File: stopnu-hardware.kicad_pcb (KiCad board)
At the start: 4 copper layers, 150 x 128 mm, 48 parts, among them CN1 SM04B-SRSS-TB (LF)(SN), CN2 OQ0232510000G, CN3 OQ0232510000G, CN4 OQ0232510000G, U1 WIFI_KIT_32__V3_, U2 74HCT1G125GW-Q100H, U5 LTV-817S, U6 LTV-817S, U7 LTV-817S

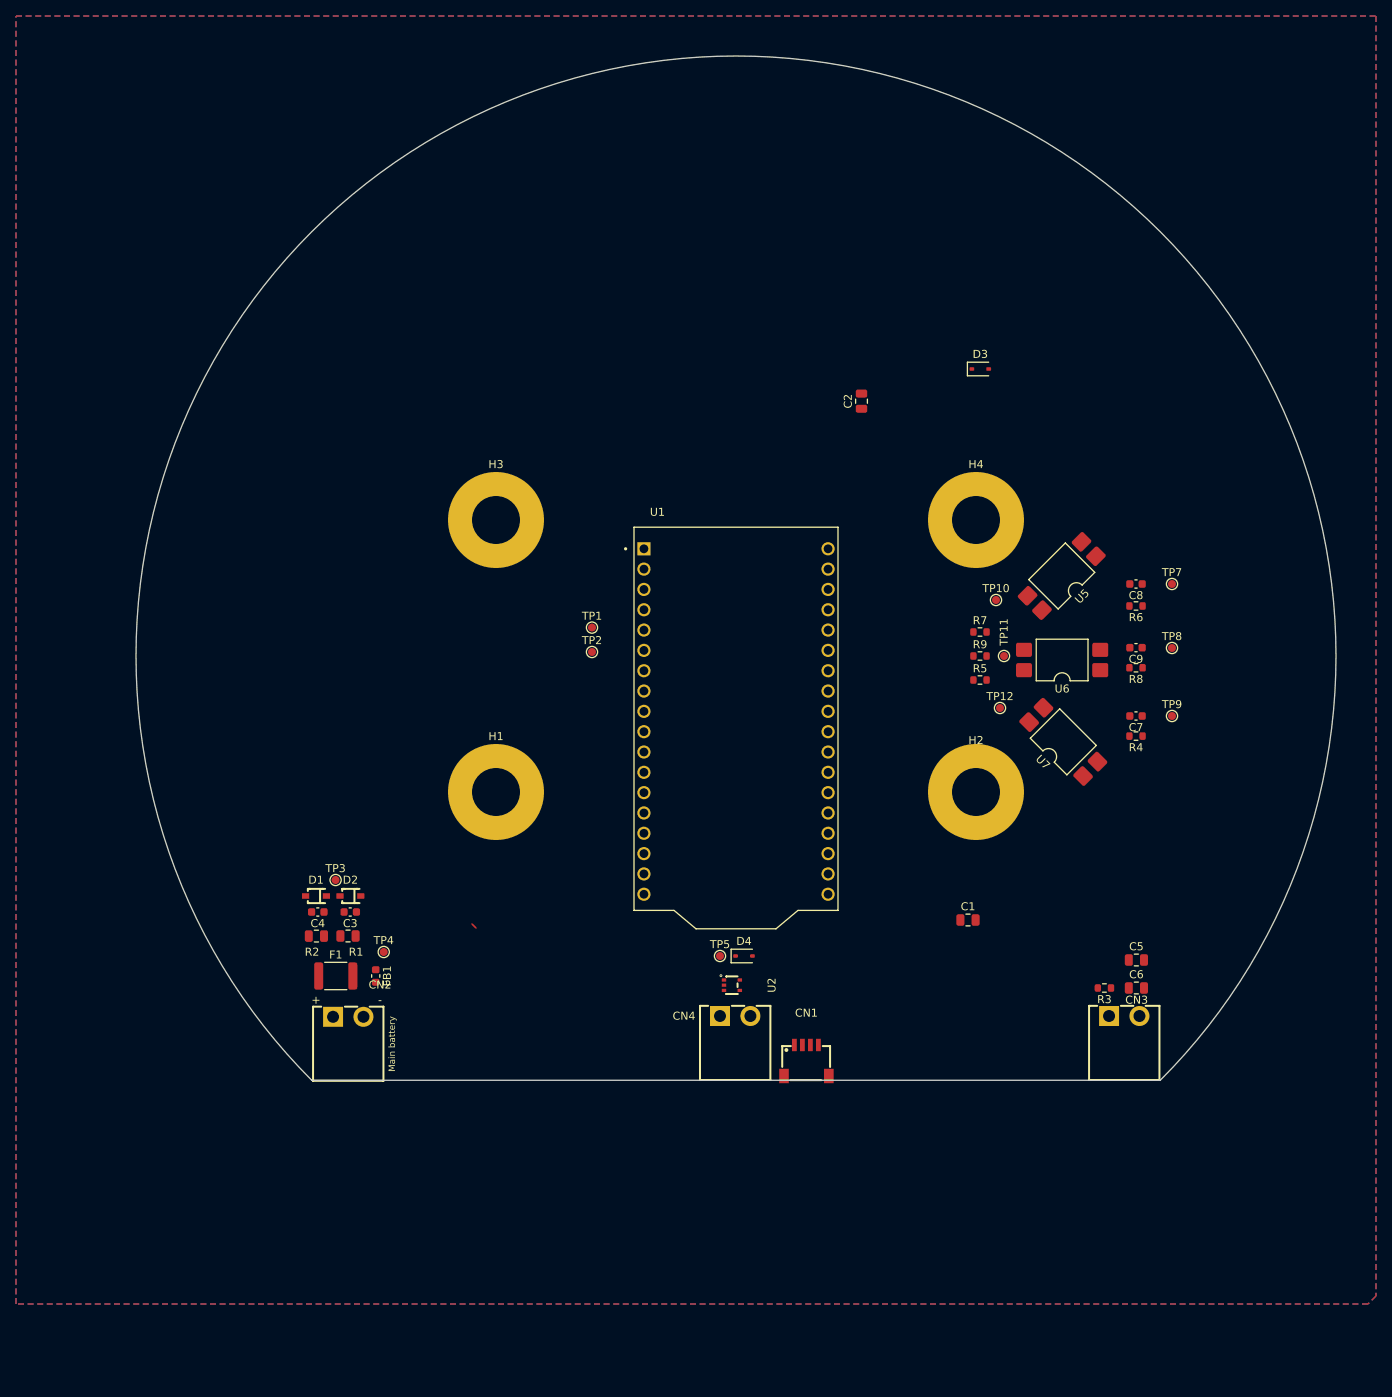
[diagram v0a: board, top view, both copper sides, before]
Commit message: Push schematic stuff missed before.
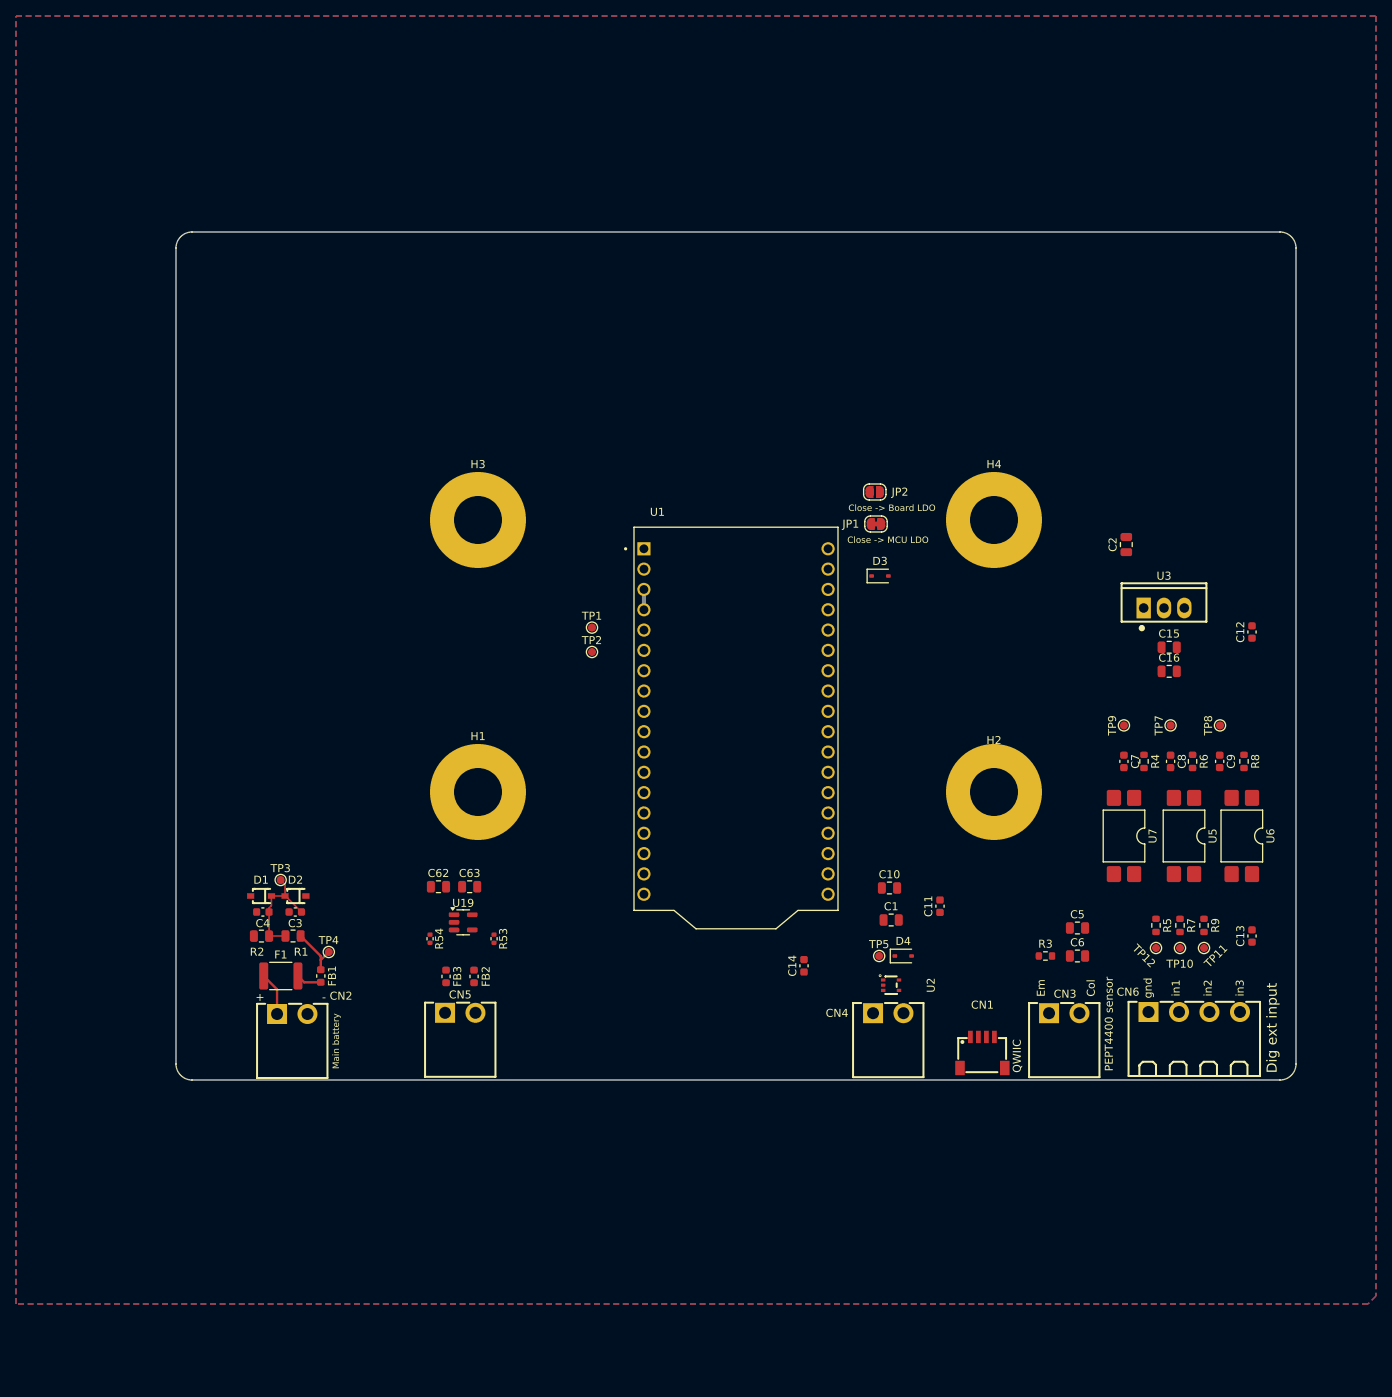
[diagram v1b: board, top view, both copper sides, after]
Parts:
- added C10: 100nF, Capacitor_SMD:C_0805_2012Metric, F.Cu at (19.2, 29.0)
- added C11: C_Small, Capacitor_SMD:C_0603_1608Metric, F.Cu at (25.5, 31.3)
- added C12: C_Small, Capacitor_SMD:C_0603_1608Metric, F.Cu at (64.5, -3.00)
- added C13: C_Small, Capacitor_SMD:C_0603_1608Metric, F.Cu at (64.5, 35.0)
- added C14: C_Small, Capacitor_SMD:C_0603_1608Metric, F.Cu at (8.50, 38.7)
- added C15: 10u, Capacitor_SMD:C_0805_2012Metric, F.Cu at (54.1, -1.09)
- added C16: 100nF, Capacitor_SMD:C_0805_2012Metric, F.Cu at (54.1, 1.92)
- added C62: 10u, Capacitor_SMD:C_0805_2012Metric, F.Cu at (-37.2, 28.8)
- added C63: 10u, Capacitor_SMD:C_0805_2012Metric, F.Cu at (-33.3, 28.8)
- added CN5: OQ0232510000G, lcsc:CONN-TH_OQ0232510000G, F.Cu at (-34.5, 44.6)
- added CN6: OQ0432510000G, lcsc:CONN-TH_4P-P3.81_OQ0432510000G, F.Cu at (57.3, 44.5)
- added FB2: BLM18PG121SN1D, Inductor_SMD:L_0603_1608Metric, F.Cu at (-32.7, 40.1)
- added FB3: BLM18PG121SN1D, Inductor_SMD:L_0603_1608Metric, F.Cu at (-36.2, 40.1)
- added JP1: Jumper_2_Bridged, Jumper:SolderJumper-2_P1.3mm_Bridged_RoundedPad1.0x1.5mm, F.Cu at (17.5, -16.5)
- added JP2: Jumper_2_Open, Jumper:SolderJumper-2_P1.3mm_Open_RoundedPad1.0x1.5mm, F.Cu at (17.4, -20.5)
- added R53: 10k, Resistor_SMD:R_0402_1005Metric, F.Cu at (-30.2, 35.3)
- added R54: 6.8k, Resistor_SMD:R_0402_1005Metric, F.Cu at (-38.2, 35.3)
- added U19: SY6280AAC, Package_TO_SOT_SMD:SOT-23-5, F.Cu at (-34.1, 33.3)
- added U3: LD1117V33, lcsc:TO-220-3_L10.0-W4.5-P2.54-L, F.Cu at (53.5, -6.00)
- FB1: value FerriteBead_Small -> BLM18PG121SN1D
- moved TP10 49.2 mm to (55.5, 36.5)
- moved R7 44.4 mm to (55.5, 33.7), turned to -90 degrees
- moved TP11 44.2 mm to (58.5, 36.5), turned to 180 degrees
- moved R9 43.8 mm to (58.5, 33.7), turned to -90 degrees
- moved R5 37.7 mm to (52.5, 33.7), turned to -90 degrees
- moved C2 37.6 mm to (48.8, -13.9)
- moved U5 35.9 mm to (56.0, 22.5), turned to -90 degrees
- moved TP12 35.8 mm to (52.5, 36.5), turned to 135 degrees
- moved U6 31.4 mm to (63.2, 22.5), turned to -90 degrees
- moved D3 28.8 mm to (18.0, -10.0)
- moved C8 22.6 mm to (54.3, 13.2), turned to -90 degrees
- moved CN1 22.0 mm to (30.8, 49.6)
- moved R6 20.7 mm to (57.1, 13.2), turned to -90 degrees
- moved D4 19.9 mm to (20.9, 37.5)
- moved TP5 19.9 mm to (17.9, 37.5)
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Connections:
- D3 pad 1: +3.3V -> +3V3
- U1 pad J3_2: +3V3 -> /MCU/+3V3MCU
- U1 pad J3_3: +3V3 -> /MCU/+3V3MCU
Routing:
- net /battery_50v_to_adc/VBATT_LVL_OUT_LOW: track 0.00 -> 14.0 mm
- net /battery_50v_to_adc/VBATT_3_V50: track 0.00 -> 6.67 mm
- net /battery_50v_to_adc/VBATT_V50: track 0.00 -> 5.44 mm
- net /battery_50v_to_adc/VBATT_2_V50: track 0.00 -> 3.19 mm
- net VBATT: track 0.00 -> 2.54 mm
- net (no net): track 0.71 -> 0.00 mm
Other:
- board size 150 x 128 mm -> 140 x 106 mm
- board text added: "Bracket housing stay out"

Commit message: Some extra work for building the rats nest.
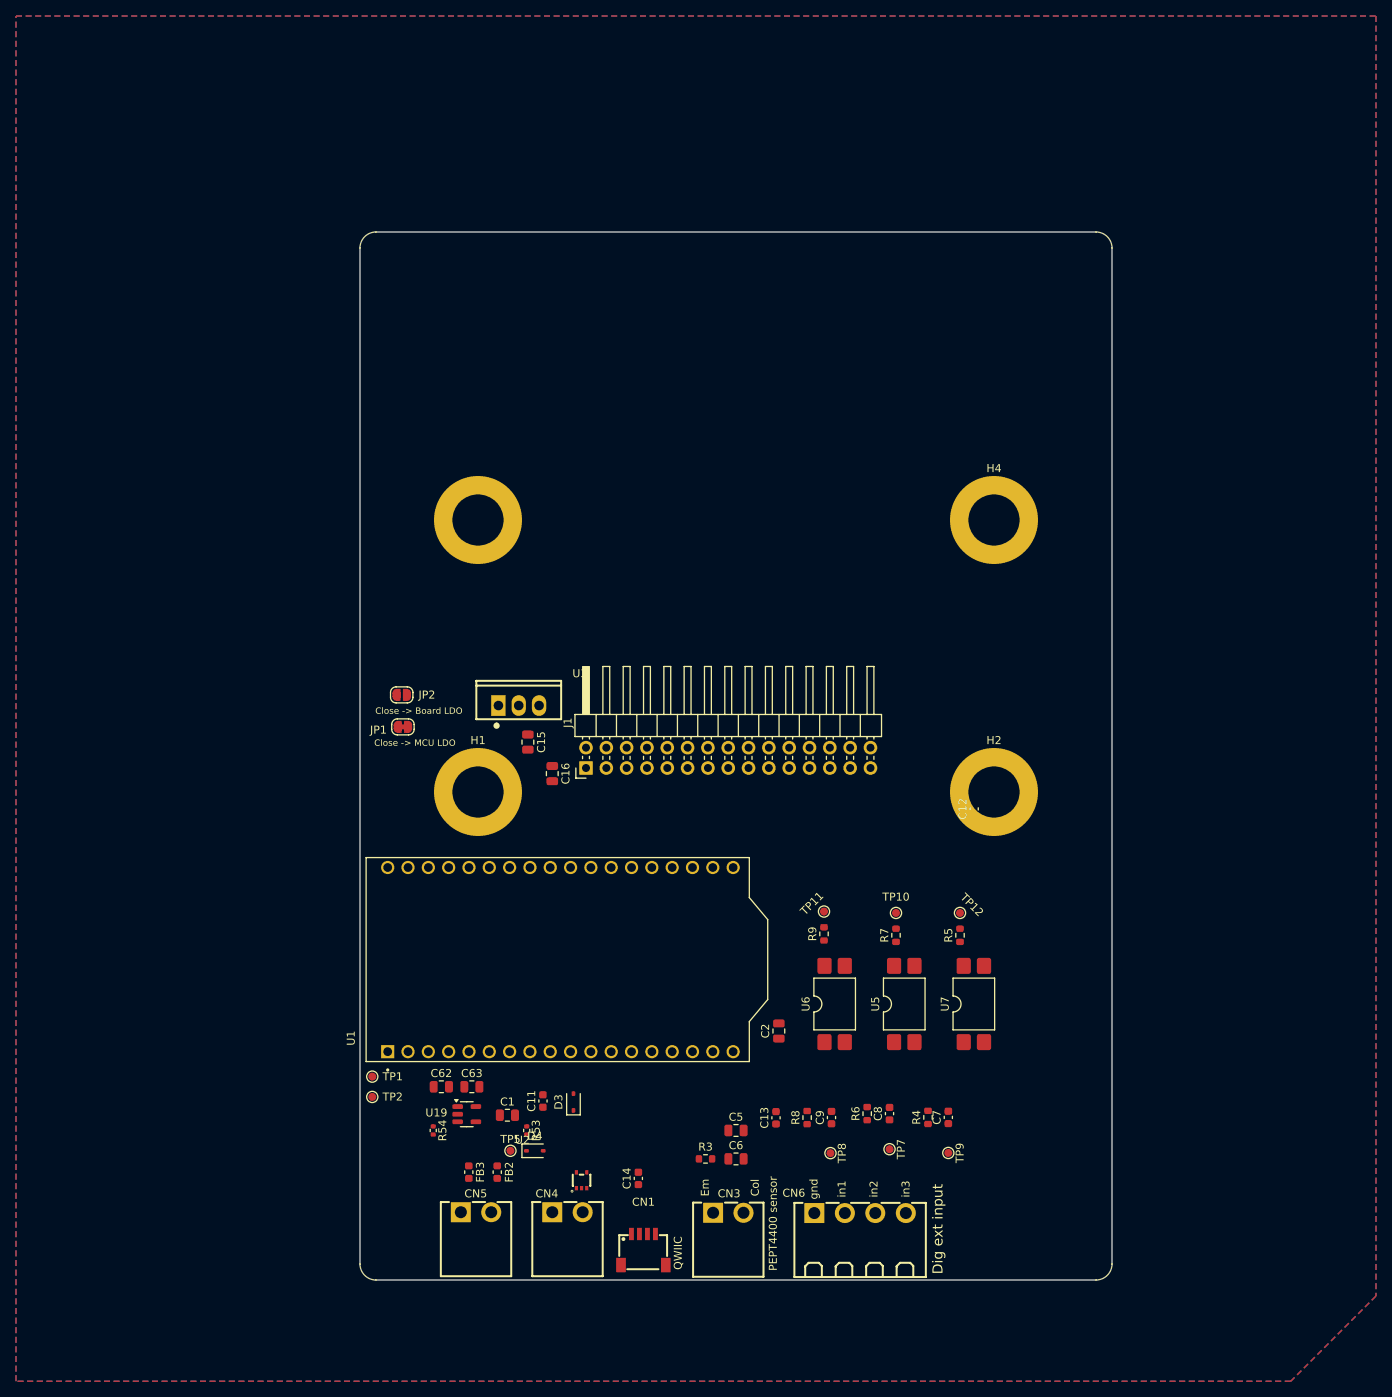
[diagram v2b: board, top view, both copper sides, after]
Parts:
- removed C10: 100nF, Capacitor_SMD:C_0805_2012Metric
- removed C3, C4: 10nF, Capacitor_SMD:C_0603_1608Metric
- removed CN2: OQ0232510000G, lcsc:CONN-TH_OQ0232510000G
- removed D1, D2: 1N4148WSG_C2904852, lcsc:SOD-323_L1.6-W1.3-LS2.7-RD
- removed F1: Polyfuse, Fuse:Fuse_1812_4532Metric
- removed FB1: BLM18PG121SN1D, Inductor_SMD:L_0603_1608Metric
- removed R1: 100k, Capacitor_SMD:C_0805_2012Metric
- removed R2: 3.6K, Capacitor_SMD:C_0805_2012Metric
- removed TP3, TP4: TestPoint, TestPoint:TestPoint_Pad_D1.0mm
- added J1: Conn_02x15_Odd_Even, Connector_PinHeader_2.54mm:PinHeader_2x15_P2.54mm_Horizontal, F.Cu at (-18.8, 14.0)
- H1, H2, H3, H4: footprint MountingHole:MountingHole_6mm_Pad -> MountingHole:MountingHole_6.4mm_M6_DIN965_Pad
- moved U3 81.6 mm to (-27.2, 6.19)
- moved C15 81.0 mm to (-26.0, 10.8), turned to -90 degrees
- moved C16 78.2 mm to (-23.0, 14.7), turned to -90 degrees
- moved D3 76.1 mm to (-20.3, 55.8), turned to 90 degrees
- moved C2 74.7 mm to (5.36, 46.9)
- moved TP8 72.3 mm to (11.8, 62.1), turned to -90 degrees
- moved R8 70.5 mm to (8.89, 57.7), turned to 90 degrees
- moved C9 65.9 mm to (11.9, 57.7), turned to 90 degrees
- moved JP1 64.3 mm to (-41.6, 8.86)
- moved JP2 64.3 mm to (-41.8, 4.86)
- moved C13 63.7 mm to (5.00, 57.7)
- moved TP7 63.6 mm to (19.2, 61.6), turned to -90 degrees
- moved TP1 62.5 mm to (-45.5, 52.6), turned to -90 degrees
- moved TP2 62.0 mm to (-45.5, 55.1), turned to -90 degrees
- moved R6 59.9 mm to (16.4, 57.2), turned to 90 degrees
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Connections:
- net /MCU/GPIO33 renamed /GPIO42
- net /MCU/MCU_VBAT_3V3 renamed /HELTEC V3/MCU_VBAT_3V3
- net Net-(U1A-U0RXD/GPIO44/CP2102_TX) renamed /UART_TX
- net Net-(U1A-U0TXD/GPIO43/CP2102_RX) renamed /UART_RX
- CN1 pad 3: /QWIIC_SDA -> /GPIO47
- CN1 pad 4: /QWIIC_SCL -> /GPIO48
- CN6 pad 2: /Button IO/BUT_OUT_01 -> /Button IO/BUT_IN_03
- CN6 pad 3: /Button IO/BUT_OUT_02 -> /Button IO/BUT_IN_02
- CN6 pad 4: /Button IO/BUT_OUT_03 -> /Button IO/BUT_IN_01
- JP1 pad 2: /MCU/+3V3MCU -> +3V3
- R5 pad 2: /Button IO/BUT_OUT_01 -> /GPIO5
- R7 pad 2: /Button IO/BUT_OUT_02 -> /GPIO6
- R9 pad 2: /Button IO/BUT_OUT_03 -> /GPIO7
- TP10 pad 1: /Button IO/BUT_OUT_02 -> /GPIO6
- TP11 pad 1: /Button IO/BUT_OUT_03 -> /GPIO7
- TP12 pad 1: /Button IO/BUT_OUT_01 -> /GPIO5
- U1 pad J2_10: unconnected-(U1A-GPIO20/U1CTS/ADC2_CH9/CLK_OUT1/USB_D+-PadJ2_10) -> /USB_D+
- U1 pad J2_11: unconnected-(U1A-GPIO19/U1RST/ADC2_CH9/CLK_OUT2/USB_D--PadJ2_11) -> /USB_D-
- U1 pad J2_12: /MCU/GPIO07 -> /GPIO33
- U1 pad J2_13: /MCU/GPIO06 -> /GPIO47
- U1 pad J2_14: /MCU/GPIO05 -> /GPIO48
- U1 pad J2_15: /MCU/GPIO04 -> /GPIO26
- U1 pad J2_7: /MCU/MCU_RST -> /MCU_RST
- U1 pad J2_8: unconnected-(U1A-GPIO0/USER_SW-PadJ2_8) -> /USER_KEY
- U1 pad J2_9: unconnected-(U1A-GPIO21/OLED_RST-PadJ2_9) -> /OLED_RST
- U1 pad J3_10: /MCU/GPIO36 -> /GPIO39
- U1 pad J3_11: /MCU/GPIO37 -> /GPIO38
- U1 pad J3_12: unconnected-(U1B-GPIO38/FSPIWP/SUBSPIWP-PadJ3_12) -> /GPIO01
- U1 pad J3_13: unconnected-(U1B-GPIO39/MTCK-PadJ3_13) -> /GPIO02
- U1 pad J3_14: unconnected-(U1B-GPIO40/MTDO-PadJ3_14) -> /GPIO03
- U1 pad J3_15: unconnected-(U1B-GPIO41/MTDI-PadJ3_15) -> /GPIO04
- U1 pad J3_16: unconnected-(U1B-GPIO42/MTMS-PadJ3_16) -> /GPIO05
- U1 pad J3_17: /MCU/GPIO45 -> /GPIO06
- U1 pad J3_18: /MCU/GPIO46 -> /GPIO07
- U1 pad J3_2: /MCU/+3V3MCU -> +3V3
- U1 pad J3_3: /MCU/+3V3MCU -> +3V3
- U1 pad J3_5: /MCU/GPIO48 -> unconnected-(U1B-GPIO46-PadJ3_5)
- U1 pad J3_6: /MCU/GPIO47 -> unconnected-(U1B-GPIO45-PadJ3_6)
- U1 pad J3_8: /MCU/GPIO34 -> /GPIO41
- U1 pad J3_9: /MCU/GPIO35 -> /GPIO40
- U5 pad 4: /Button IO/BUT_OUT_02 -> /GPIO6
- U6 pad 4: /Button IO/BUT_OUT_03 -> /GPIO7
- U7 pad 4: /Button IO/BUT_OUT_01 -> /GPIO5
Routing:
- net /battery_50v_to_adc/VBATT_LVL_OUT_LOW: track 14.0 -> 0.00 mm
- net /battery_50v_to_adc/VBATT_3_V50: track 6.67 -> 0.00 mm
- net /battery_50v_to_adc/VBATT_V50: track 5.44 -> 0.00 mm
- net /battery_50v_to_adc/VBATT_2_V50: track 3.19 -> 0.00 mm
- net VBATT: track 2.54 -> 0.00 mm
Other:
- board size 140 x 106 mm -> 94 x 131 mm
- board text removed: "USB-C cable Clearance"
